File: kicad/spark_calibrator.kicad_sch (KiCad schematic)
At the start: 18 parts, among them J1 PWM, J2 Coil+, J3 Coil-, J4 12V IN, Q1 BS170, Q2 IRFP460PBF, U1 4N28

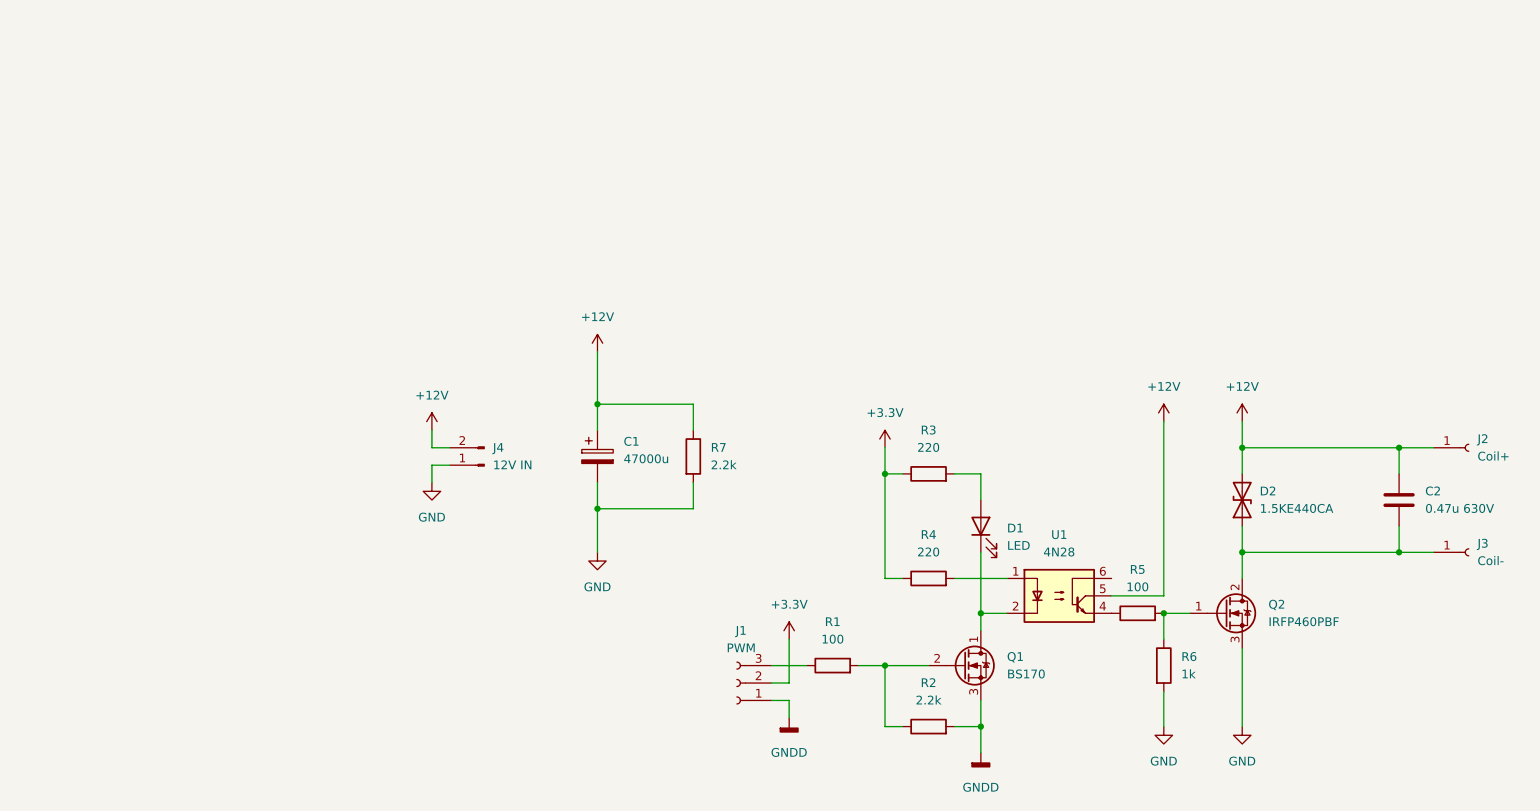
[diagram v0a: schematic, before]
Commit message: aestetic updates
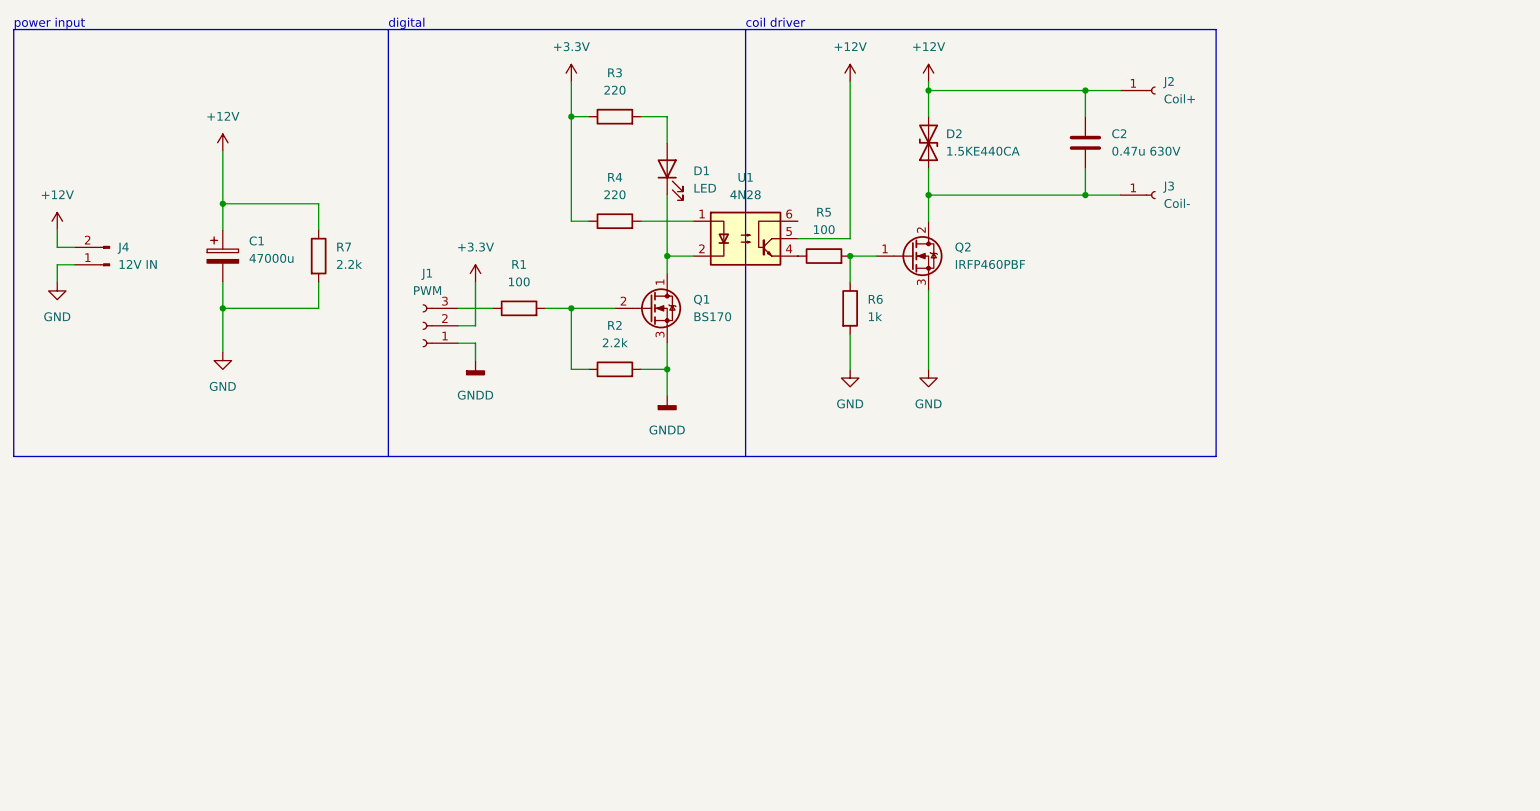
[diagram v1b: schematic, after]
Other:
- note added: "coil driver"
- note added: "digital"
- note added: "power input"
- company: (none) -> Author: felhub
- title: (none) -> spark_calibrator
- moved on the sheet: C1, C2, D1, D2, J1, J2, J3, J4, Q1, Q2, R1, R2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
